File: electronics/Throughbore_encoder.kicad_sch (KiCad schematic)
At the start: 4 parts, among them J4 Conn_01x06

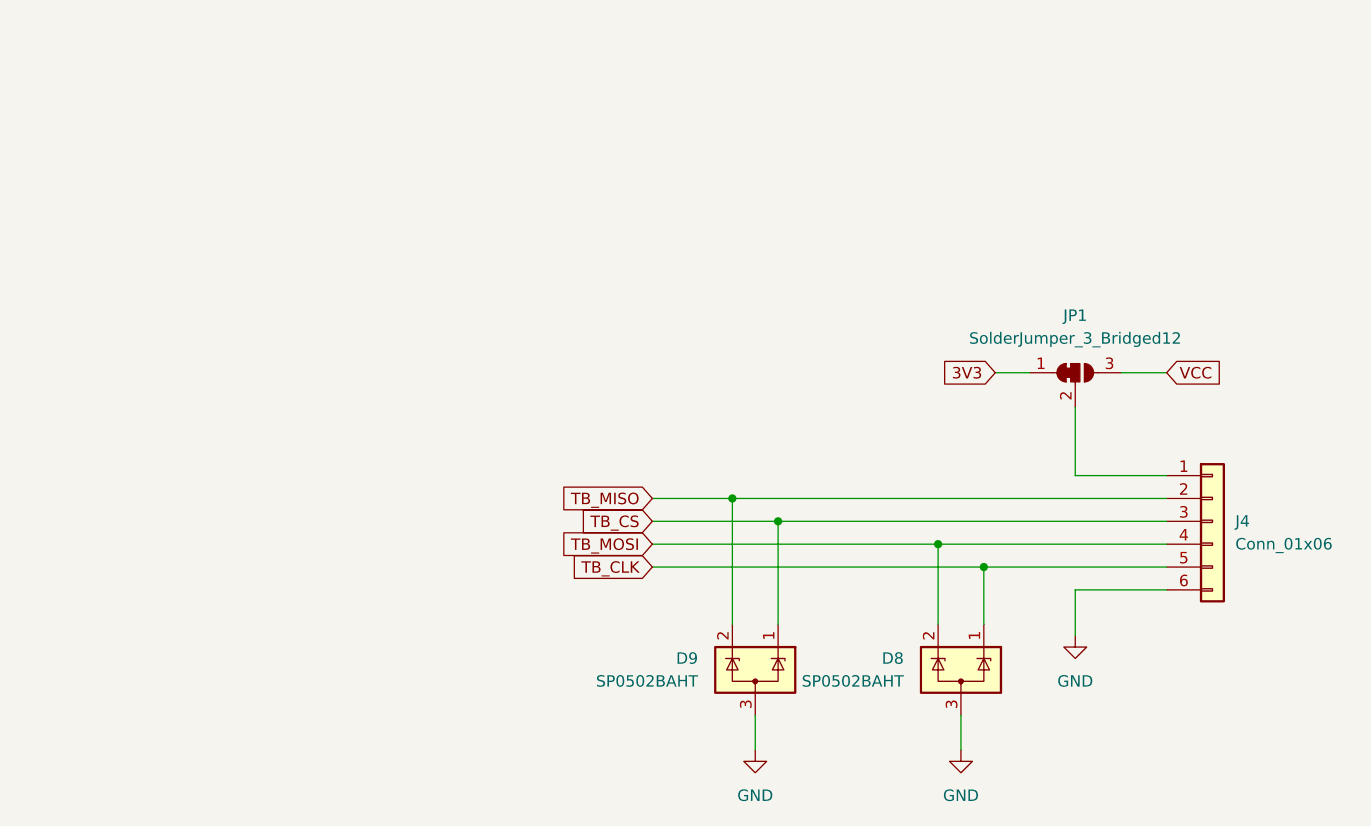
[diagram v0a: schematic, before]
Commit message: Major refactor to rev B
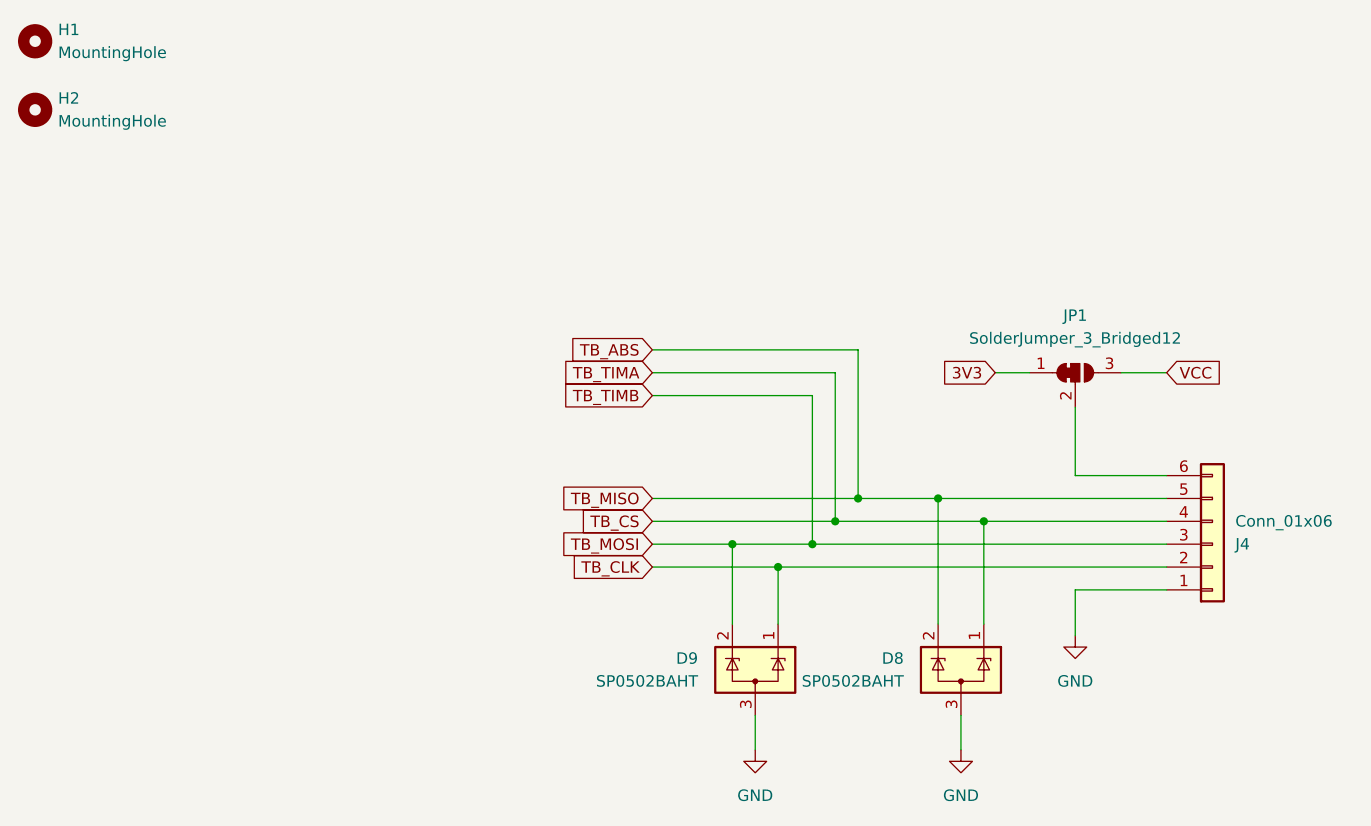
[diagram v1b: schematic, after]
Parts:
- added H1, H2: MountingHole, MountingHole:MountingHole_2.2mm_M2, symbol Mechanical:MountingHole
- J4: footprint (none) -> Connector_JST:JST_PH_S6B-PH-K_1x06_P2.00mm_Horizontal; JLCPCB (none) -> C157920
- JP1: footprint (none) -> Jumper:SolderJumper-3_P1.3mm_Bridged2Bar12_RoundedPad1.0x1.5mm_NumberLabels
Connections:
- net GND: now also J4.1 (Pin_1); no longer J4.6 (Pin_6)
- net TB_CLK: now also D9.1 (K), J4.2 (Pin_2); no longer D8.1 (K), J4.5 (Pin_5)
- net TB_CS: now also D8.1 (K), J4.4 (Pin_4); no longer D9.1 (K), J4.3 (Pin_3)
- net TB_MOSI: now also D9.2 (K), J4.3 (Pin_3); no longer D8.2 (K), J4.4 (Pin_4)
- net at JP1.2 (C): now also J4.6 (Pin_6); no longer J4.1 (Pin_1)
- removed net TB_MISO: D9.2 (K), J4.2 (Pin_2)
- new net TB_ABS: D8.2 (K), J4.5 (Pin_5)
